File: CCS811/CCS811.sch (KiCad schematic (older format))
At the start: 26 parts, among them J1 Conn_01x04, J2 Conn_01x04, Q1 BSS138DW, Q2 BSS138, Q3 BSS138DW, U1 AP2127K-3.3, U2 CCS811

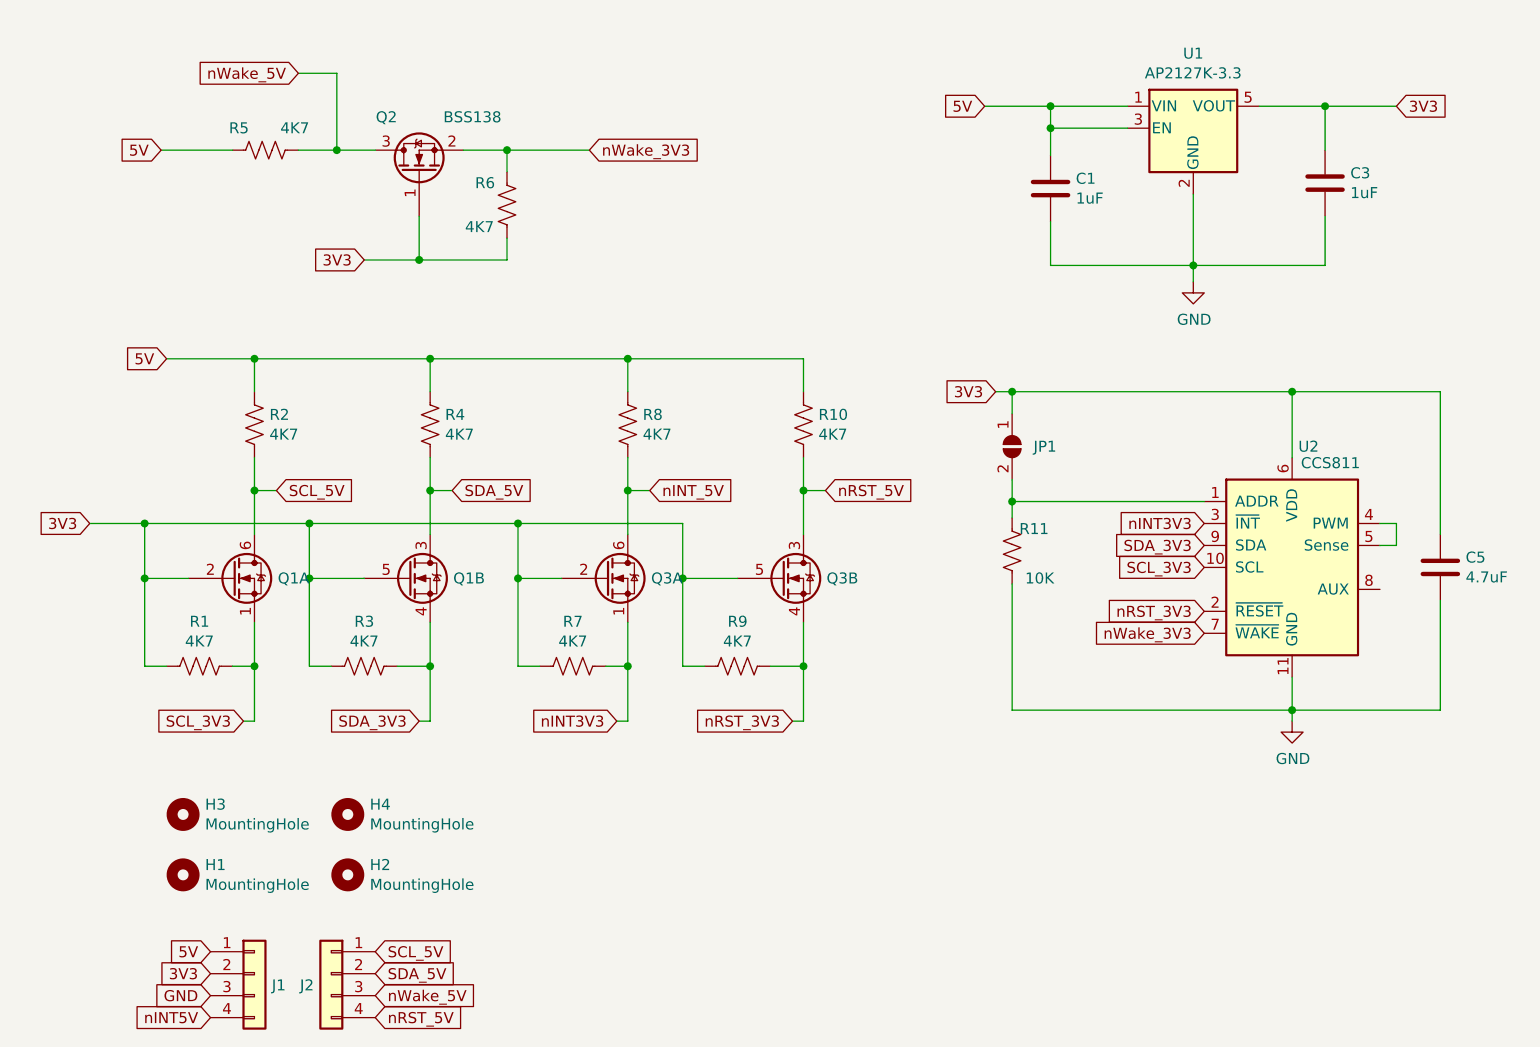
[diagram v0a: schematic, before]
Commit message: Minor Layout Updates
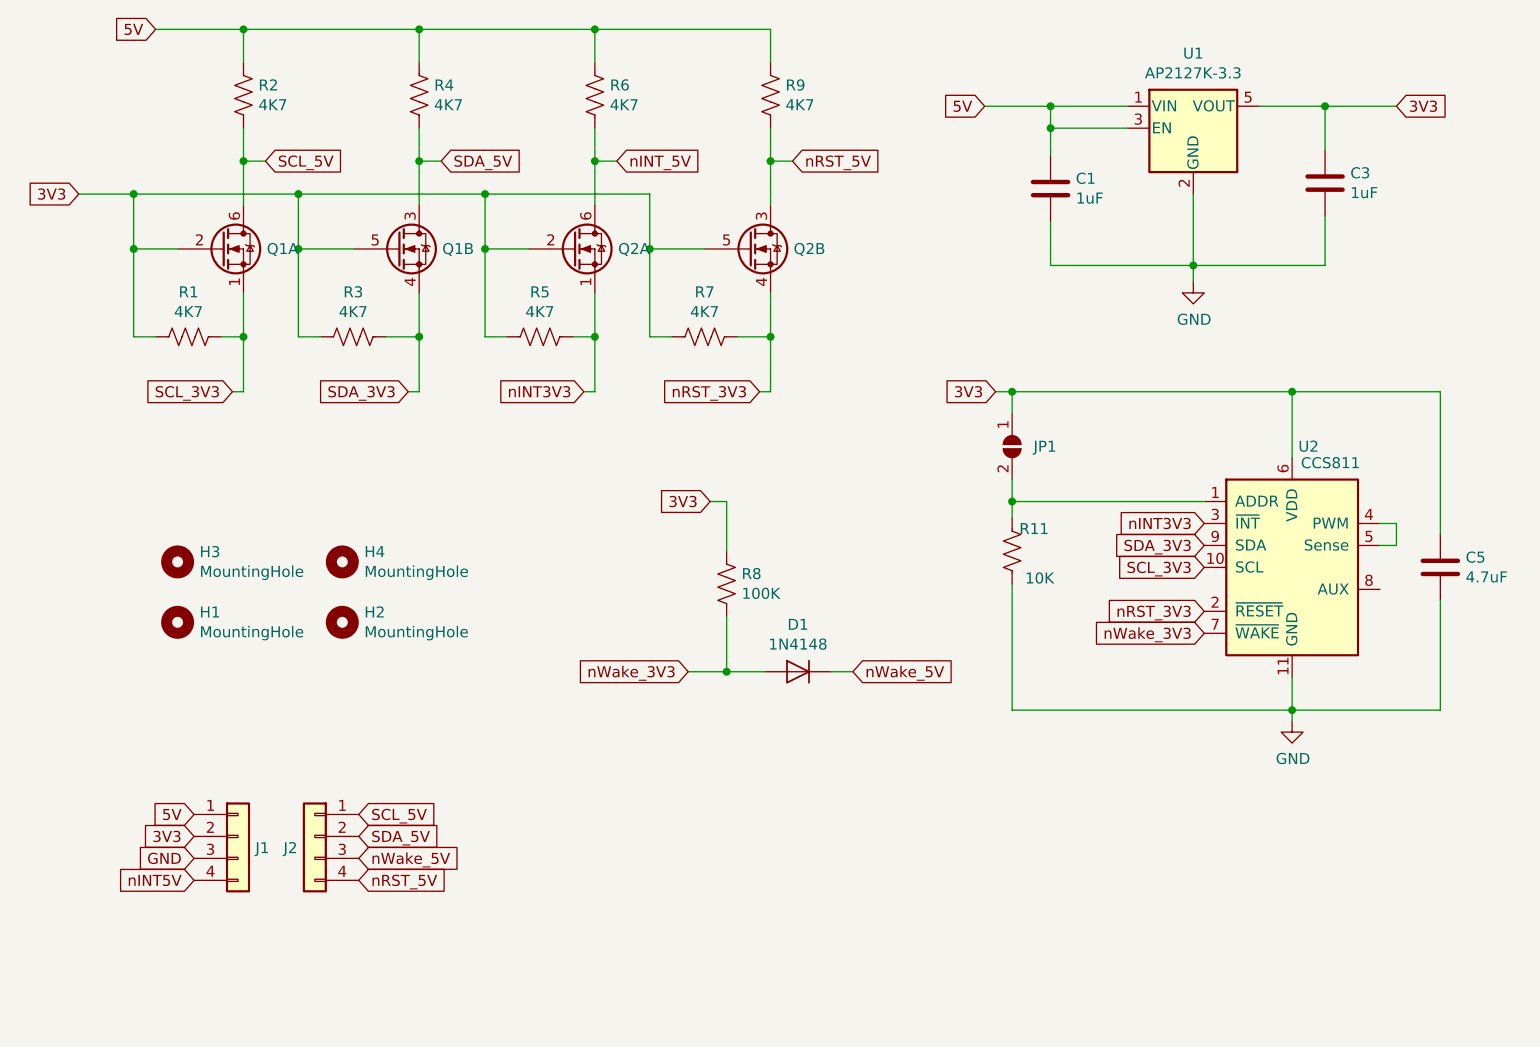
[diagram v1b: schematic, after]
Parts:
- removed Q2: BSS138, Package_TO_SOT_SMD:SOT-23, symbol Transistor_FET:BSS138
- removed Q3: BSS138DW, Package_TO_SOT_SMD:SOT-363_SC-70-6, symbol Device:Q_DUAL_NMOS_S1G1D2S2G2D1
- removed R10: 4K7, Resistor_SMD:R_0603_1608Metric, symbol Device:R_US
- added D1: 1N4148, Diode_SMD:D_SOD-523, symbol Device:D
- added Q2: BSS138DW, Package_TO_SOT_SMD:SOT-363_SC-70-6, symbol Device:Q_DUAL_NMOS_S1G1D2S2G2D1
- R8: value 4K7 -> 100K; Part C99782 -> C14675
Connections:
- net 3V3: now also R5.2, R8.1, Q2.2 (G), Q2.5 (G); no longer R6.2, R9.2
- net 5V: now also R6.1, R9.1; no longer R5.1, R8.1
- net nINT3V3: now also R5.1, Q2.1 (S); no longer R7.1
- net nINT_5V: now also R6.2, Q2.6 (D); no longer R8.2
- net nRST_3V3: now also R7.1, Q2.4 (S); no longer R9.1
- net nRST_5V: now also R9.2, Q2.3 (D)
- net nWake_3V3: now also R8.2, D1.2 (A); no longer R6.1
- net nWake_5V: now also D1.1 (K); no longer R5.2
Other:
- moved on the sheet: H1, H2, H3, H4, J1, J2, Q1A, Q1B, R1, R2, R3, R4
